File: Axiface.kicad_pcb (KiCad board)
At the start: 2 copper layers, 55.4 x 36.3 mm, 30 parts, among them J1 Conn_01x02, J10 Conn_01x03, J11 Conn_01x04, J2 Conn_01x03, J3 Conn_01x03, J4 Conn_01x03, J5 Conn_01x03, J6 Conn_01x03, J7 Conn_01x03, J8 Conn_01x03, J9 Conn_01x03, U1 MCP1804x-5002xDB, U2 74HC241, U3 TSR_2-2490, U4 TSR_2-2490, U5 TSR_2-2490

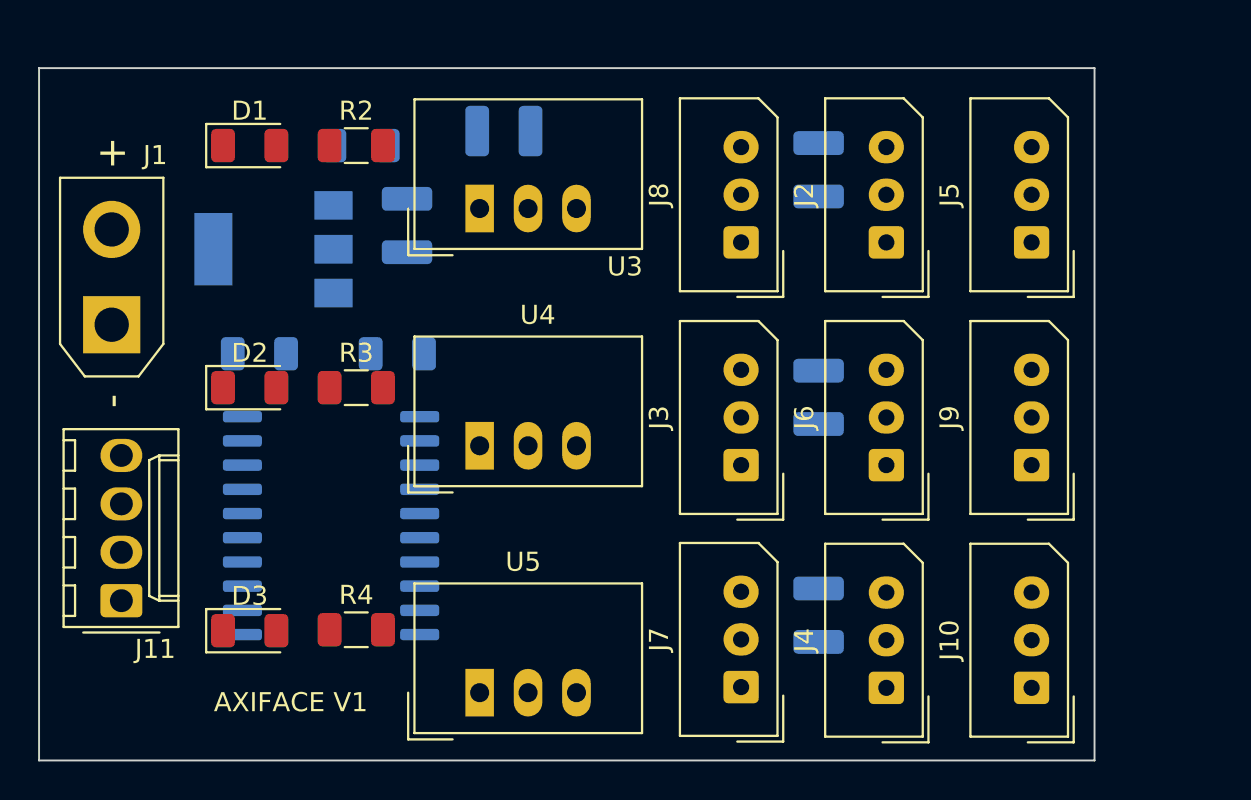
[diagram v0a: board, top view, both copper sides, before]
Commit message: Mise à jour du schéma et pcb
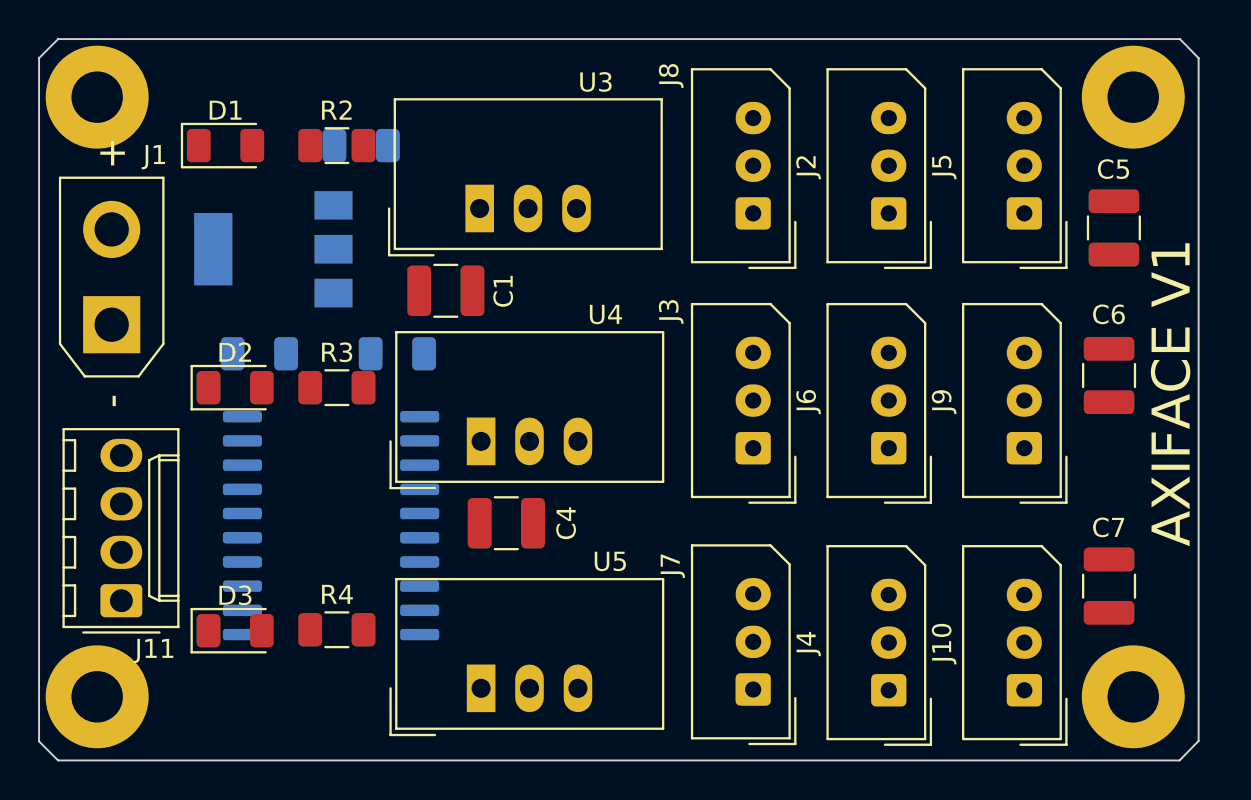
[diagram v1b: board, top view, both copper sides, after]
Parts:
- added H1: MountingHole_Pad, MountingHole:MountingHole_2.7mm_M2.5_Pad, F.Cu at (91.7, 132.3)
- added H2: MountingHole_Pad, MountingHole:MountingHole_2.7mm_M2.5_Pad, F.Cu at (91.7, 100.8)
- added H3: MountingHole_Pad, MountingHole:MountingHole_2.7mm_M2.5_Pad, F.Cu at (146.1, 100.8)
- added H4: MountingHole_Pad, MountingHole:MountingHole_2.7mm_M2.5_Pad, F.Cu at (146.1, 132.3)
- C1, C4, C5, C6, C7: moved to F.Cu
- U3, U4, U5: footprint Converter_DCDC:Converter_DCDC_TRACO_TSR-1_THT -> Convert_DCDC:Converter_DCDC_TRACO_TSR-2_THT
- moved C4 20.6 mm to (113.2, 123.2)
- moved C5 15.8 mm to (145.0, 107.7), turned to 270 degrees
- moved C7 15.3 mm to (144.8, 126.5)
- moved C6 15.3 mm to (144.8, 115.4)
- moved C1 3.98 mm to (110.0, 111.0), turned to 0 degrees
- moved J8 1.65 mm to (126.1, 106.9)
- moved J5 1.57 mm to (140.3, 106.9)
- moved J2 1.53 mm to (133.2, 106.9)
- moved D1 1.27 mm to (98.4, 103.4)
- moved J3 1.09 mm to (126.1, 119.3)
- moved R2 1.02 mm to (104.3, 103.4)
- moved R3 1.02 mm to (104.3, 116.1)
- moved R4 1.02 mm to (104.3, 128.8)
- moved J9 0.97 mm to (140.3, 119.3)
- moved J6 0.90 mm to (133.2, 119.3)
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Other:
- board size 55.4 x 36.3 mm -> 60.8 x 37.8 mm
